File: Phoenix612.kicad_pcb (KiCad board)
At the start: 2 copper layers, 233.6 x 93.2 mm, 62 parts, among them J1 LO/BFO, J2 BFO/LO, K1 G5V-2, K2 G5V-2, T1 FT50-74 (22:4), T2 FT50-75 (18:7), T3 FT50-75 (7:18), U1 LT1253, U2 QPR_Filter, U3 SA612, U4 SA612, Y1 12 MHz, Y2 12 MHz, Y3 12 MHz, Y4 12 MHz

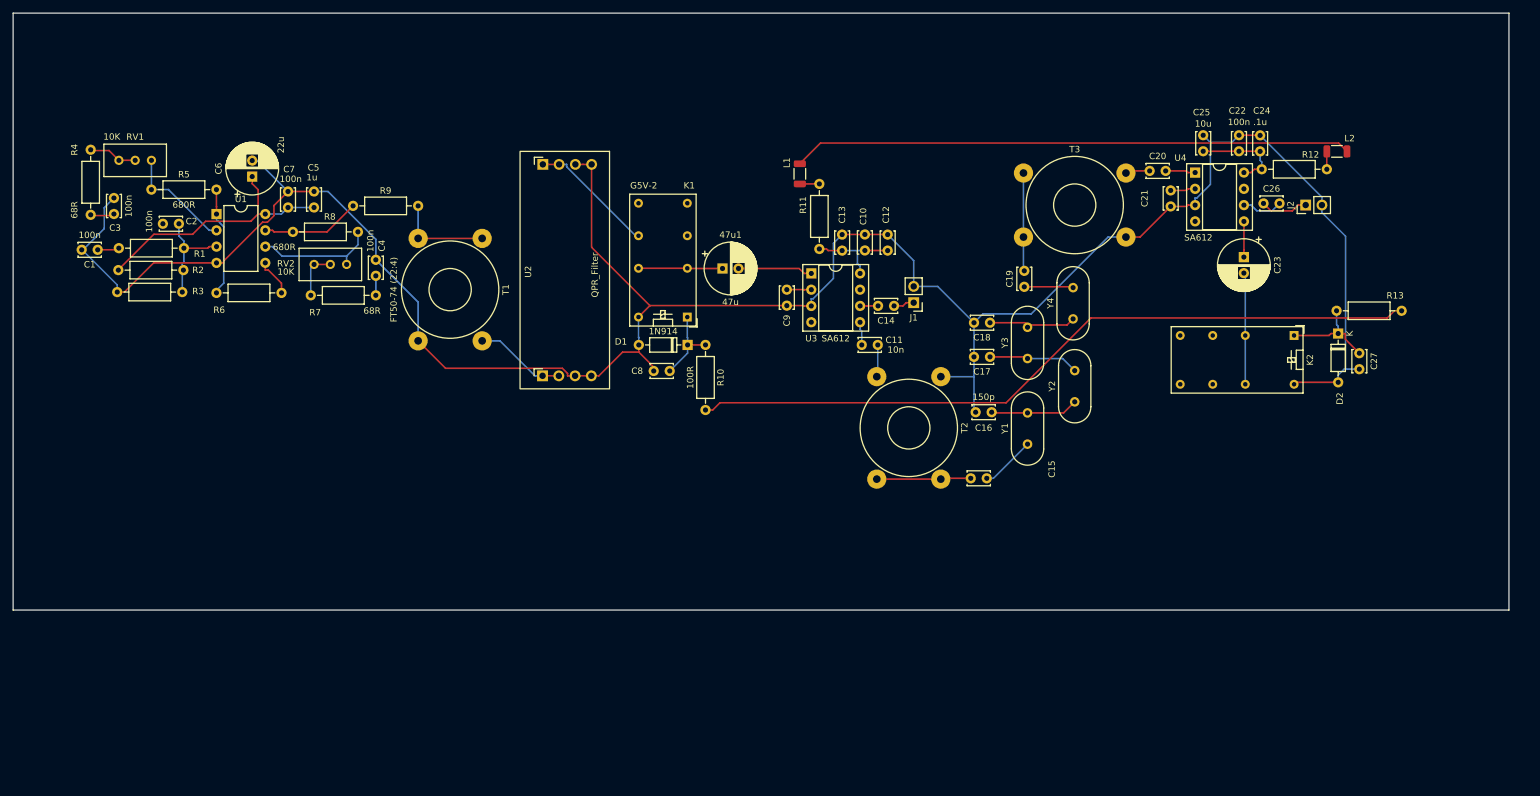
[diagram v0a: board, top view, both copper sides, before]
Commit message: Add AF Stage
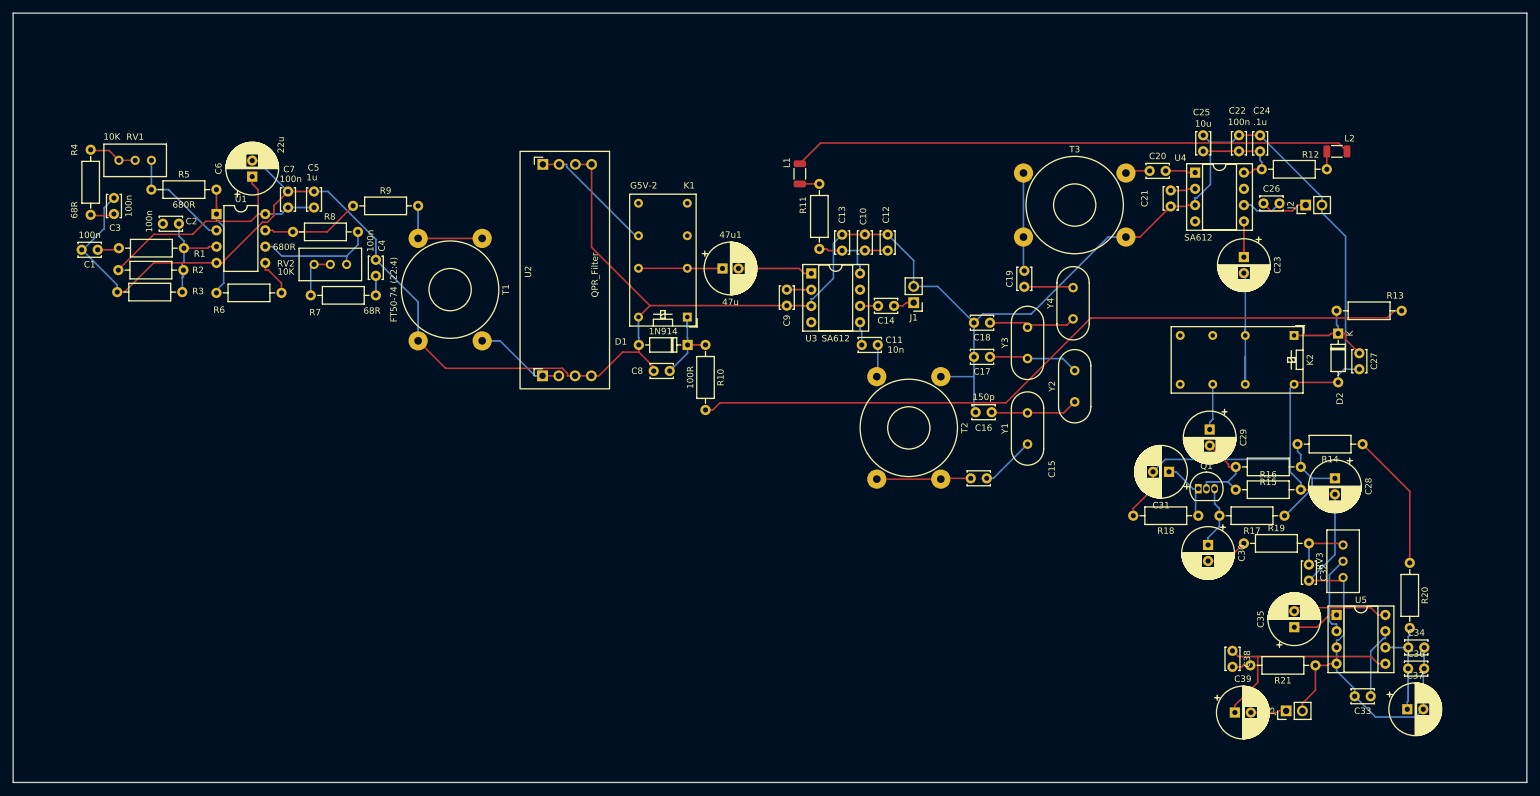
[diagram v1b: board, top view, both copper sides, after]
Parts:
- added C28: 47u, Capacitor_THT:CP_Radial_D8.0mm_P2.50mm, F.Cu at (225.0, 113.8)
- added C29: 47u, Capacitor_THT:CP_Radial_D8.0mm_P2.50mm, F.Cu at (205.5, 106.2)
- added C30: 47u, Capacitor_THT:CP_Radial_D8.0mm_P2.50mm, F.Cu at (205.2, 124.2)
- added C31: 100u, Capacitor_THT:CP_Radial_D8.0mm_P2.50mm, F.Cu at (199.1, 112.8)
- added C32: 10n, Capacitor_THT:C_Disc_D3.4mm_W2.1mm_P2.50mm, F.Cu at (221.0, 127.3)
- added C33: 1u, Capacitor_THT:C_Disc_D3.4mm_W2.1mm_P2.50mm, F.Cu at (230.6, 147.8)
- added C34: 100n, Capacitor_THT:C_Disc_D3.4mm_W2.1mm_P2.50mm, F.Cu at (236.5, 140.2)
- added C35: 10u, Capacitor_THT:CP_Radial_D8.0mm_P2.50mm, F.Cu at (218.7, 137.0)
- added C36: 1n, Capacitor_THT:C_Disc_D3.4mm_W2.1mm_P2.50mm, F.Cu at (236.5, 143.5)
- added C37: 220u, Capacitor_THT:CP_Radial_D8.0mm_P2.50mm, F.Cu at (236.3, 149.9)
- added C38: 10n, Capacitor_THT:C_Disc_D3.4mm_W2.1mm_P2.50mm, F.Cu at (209.0, 140.7)
- added C39: 100u, Capacitor_THT:CP_Radial_D8.0mm_P2.50mm, F.Cu at (209.4, 150.4)
- added J3: SPK, Connector_PinHeader_2.54mm:PinHeader_1x02_P2.54mm_Vertical, F.Cu at (217.4, 150.1)
- added Q1: 2N3904, Package_TO_SOT_THT:TO-92_Inline, F.Cu at (203.7, 115.4)
- added R14: 100R, Resistor_THT:R_Axial_DIN0207_L6.3mm_D2.5mm_P10.16mm_Horizontal, F.Cu at (229.4, 108.5)
- added R15: 100K, Resistor_THT:R_Axial_DIN0207_L6.3mm_D2.5mm_P10.16mm_Horizontal, F.Cu at (219.7, 112.0)
- added R16: 10K, Resistor_THT:R_Axial_DIN0207_L6.3mm_D2.5mm_P10.16mm_Horizontal, F.Cu at (209.6, 115.6)
- added R17: 1K, Resistor_THT:R_Axial_DIN0207_L6.3mm_D2.5mm_P10.16mm_Horizontal, F.Cu at (217.2, 119.6)
- added R18: 470R, Resistor_THT:R_Axial_DIN0207_L6.3mm_D2.5mm_P10.16mm_Horizontal, F.Cu at (203.7, 119.6)
- added R19: 2.7K, Resistor_THT:R_Axial_DIN0207_L6.3mm_D2.5mm_P10.16mm_Horizontal, F.Cu at (210.8, 124.0)
- added R20: 100R, Resistor_THT:R_Axial_DIN0207_L6.3mm_D2.5mm_P10.16mm_Horizontal, F.Cu at (236.7, 127.0)
- added R21: 10R, Resistor_THT:R_Axial_DIN0207_L6.3mm_D2.5mm_P10.16mm_Horizontal, F.Cu at (222.0, 143.0)
- added RV3: 10K, Potentiometer_THT:Potentiometer_Bourns_3296W_Vertical, F.Cu at (226.3, 124.2)
- added U5: LM386, Package_DIP:DIP-8_W7.62mm_Socket, F.Cu at (225.3, 135.1)
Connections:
- K2 pad 11: unconnected-(K2-Pad11) -> IFAFOUT
- K2 pad 8: unconnected-(K2-Pad8) -> IFPAOUT
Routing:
- net GND: track 378.4 -> 506.5 mm
- net Net-(C38-Pad1): track 0.00 -> 34.9 mm
- net RX12V: track 0.00 -> 21.6 mm
- net Net-(C28-Pad1): track 0.00 -> 17.5 mm
- net Net-(C34-Pad1): track 0.00 -> 16.4 mm
- net Net-(C35-Pad2): track 0.00 -> 14.9 mm
- net Net-(C29-Pad2): track 0.00 -> 14.7 mm
- net Net-(RV3-Pad2): track 0.00 -> 12.7 mm
- net Net-(C33-Pad1): track 0.00 -> 11.3 mm
- net Net-(C31-Pad1): track 0.00 -> 10.1 mm
- net Net-(C30-Pad1): track 0.00 -> 9.84 mm
- net SMeterIN: track 0.00 -> 8.76 mm
- net Net-(C35-Pad1): track 0.00 -> 7.40 mm
- net IFAFOUT: track 0.00 -> 7.26 mm
- net Net-(C30-Pad2): track 0.00 -> 6.73 mm
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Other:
- board size 233.6 x 93.2 mm -> 236.4 x 120.1 mm
